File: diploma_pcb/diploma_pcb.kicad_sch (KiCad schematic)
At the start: 22 parts, among them Q1 2SC3356, Q3 2SC3356

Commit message: changes to ard, file button reader
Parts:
- Q1, Q3: footprint 2SC3356:SOT-23_MINIMOLD_REN -> 2SC3356:SOT-23_MINIMOLD_REN-M
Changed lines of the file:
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@@
 		)
 		(instances
-			(project ""
+			(project "diploma_pcb"
 				(path "/8eade999-89f4-4618-aeea-e9238b0bd165"
 					(reference "LED1")
@@
 			)
 		)
-		(property "Footprint" "2SC3356:SOT-23_MINIMOLD_REN"
+		(property "Footprint" "2SC3356:SOT-23_MINIMOLD_REN-M"
 			(at 48.895 62.865 0)
 			(effects
@@
 			)
 		)
-		(property "Footprint" "2SC3356:SOT-23_MINIMOLD_REN"
+		(property "Footprint" "2SC3356:SOT-23_MINIMOLD_REN-M"
 			(at 48.895 62.865 0)
 			(effects

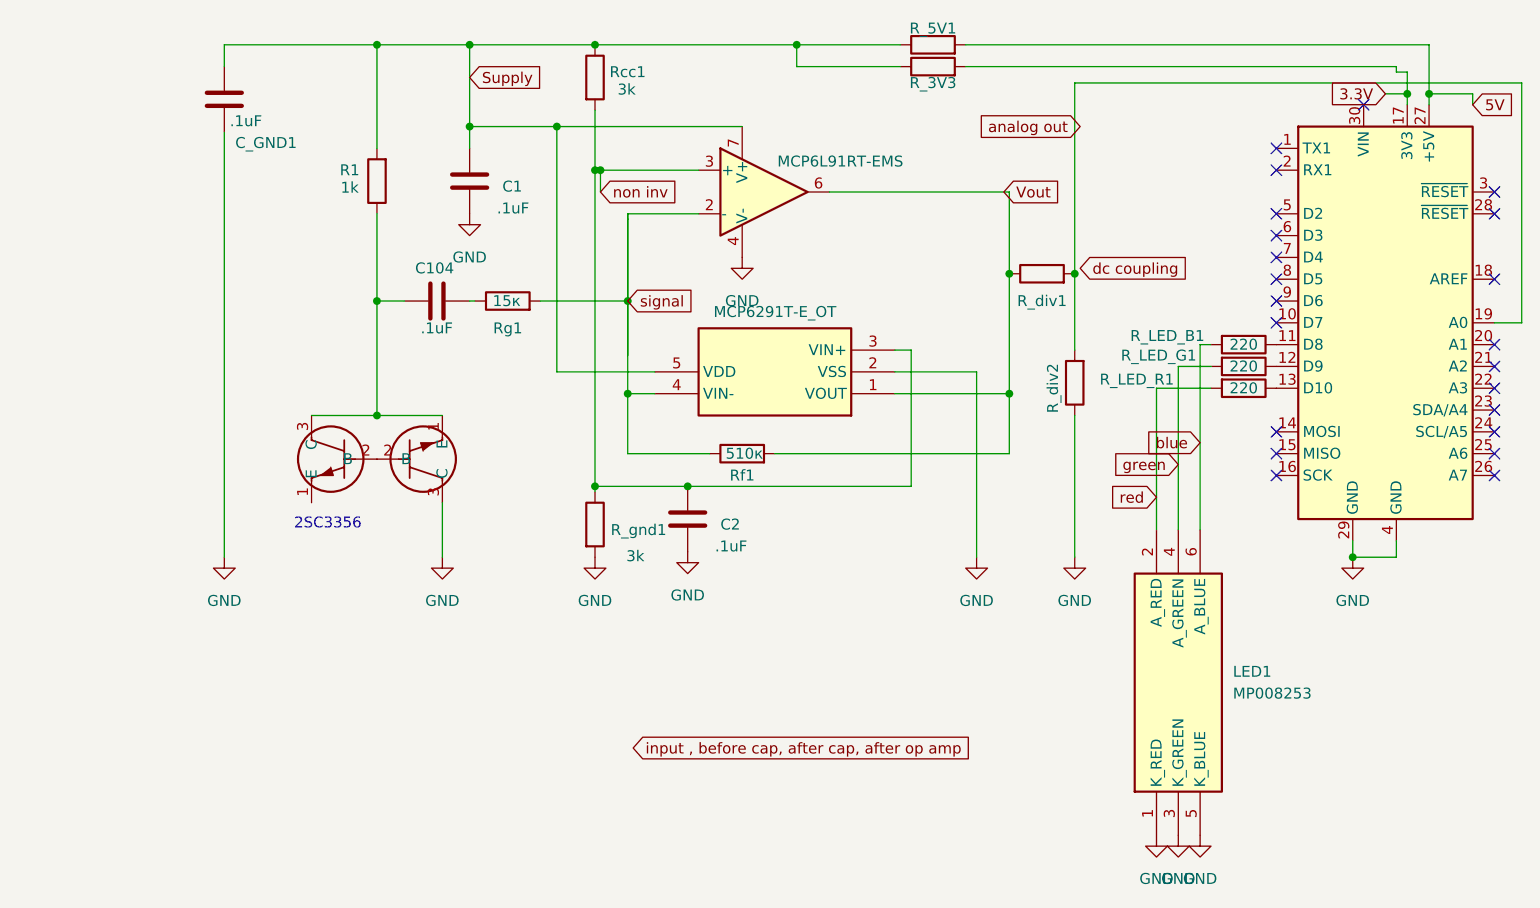
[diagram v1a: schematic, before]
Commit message: mods on PCB, Matplot, ?ard?
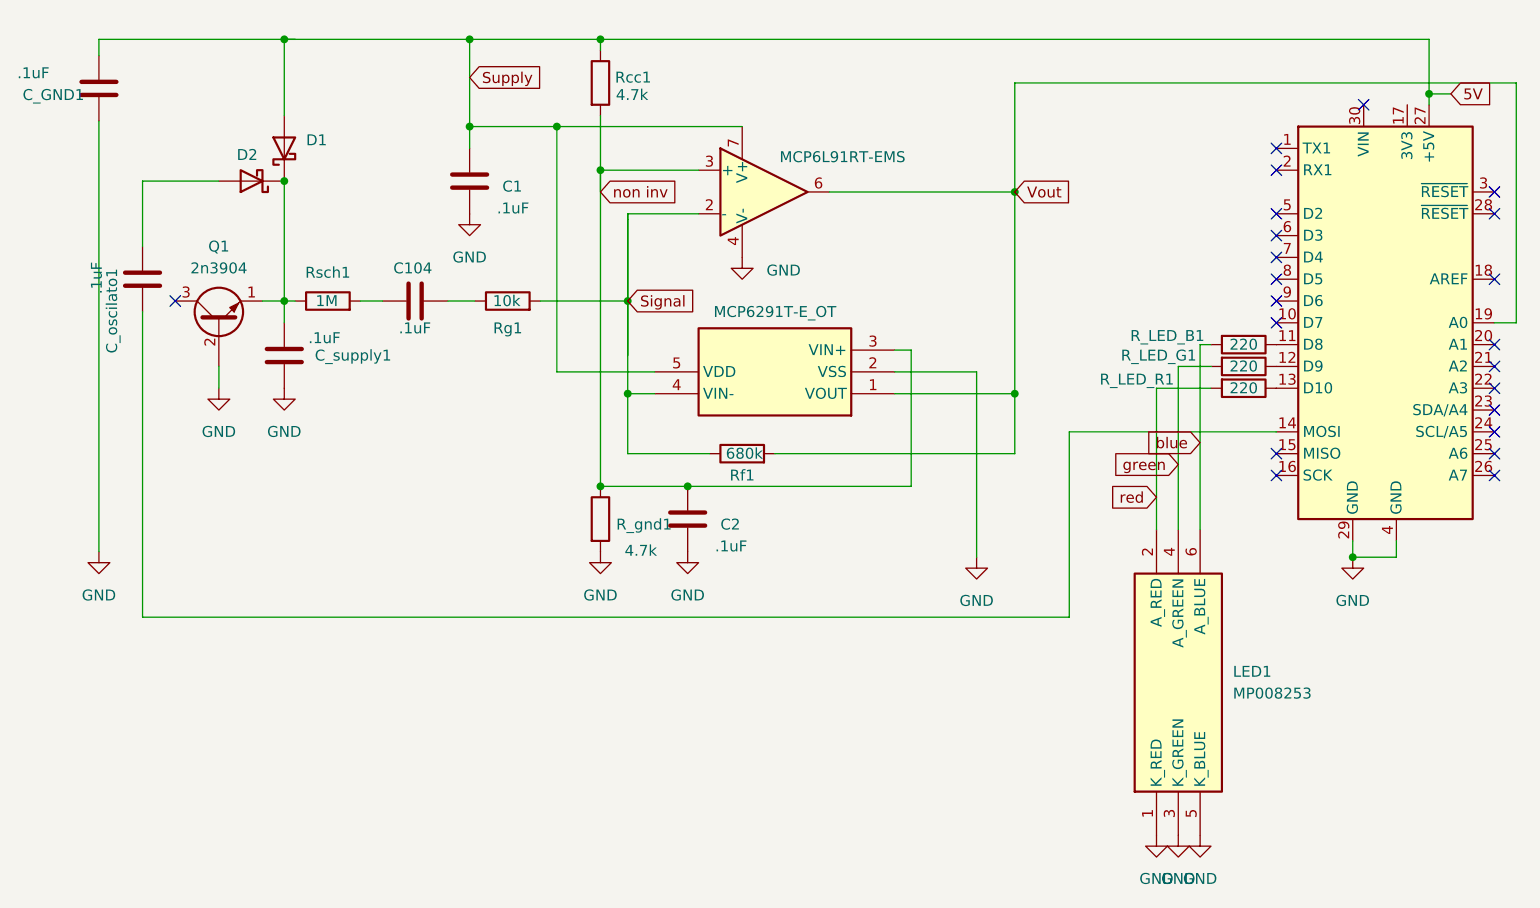
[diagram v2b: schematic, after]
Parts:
- removed Q1, Q3: 2SC3356, 2SC3356:SOT-23_MINIMOLD_REN-M, symbol 2024-08-01_13-32-15:2SC3356
- removed R1: 1k, Resistor_SMD:R_1206_3216Metric, symbol Device:R
- removed R_3V3, R_5V1, R_div1, R_div2: R, Resistor_SMD:R_1206_3216Metric, symbol Device:R
- added C_oscilato1, C_supply1: .1uF, Capacitor_SMD:C_1206_3216Metric_Pad1.33x1.80mm_HandSolder, symbol Device:C
- added D1, D2: D_Schottky, symbol Device:D_Schottky
- added Q1: 2n3904, symbol Transistor_BJT:BC107
- added Rsch1: 1M, Resistor_SMD:R_1206_3216Metric, symbol Device:R
- R_gnd1, Rcc1: value 3k -> 4.7k
- Rf1: value 510к -> 680k
- Rg1: value 15к -> 10k
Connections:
- net Supply is gone; now on net 5V: 5_pins_op_amp1.5 (VDD), 8_pin_op_amp1.7 (V+), C1.1, C_GND1.2, Rcc1.1
- net 5V: now also D1.2 (A)
- net GND: now also C_supply1.1, Q1.2 (B)
- net Vout: now also A1.19 (A0)
- net at C104.1: now also Rsch1.2
- net at A1.14 (MOSI): now also C_oscilato1.2
- net 3.3V: no longer names the net of A1.17 (3V3)
- net signal renamed Signal
- new net: C_supply1.2, D1.1 (K), D2.1 (K), Q1.1 (E), Rsch1.1
- new net: C_oscilato1.1, D2.2 (A)
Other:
- note removed: "2SC3356"
- moved on the sheet: C104, C_GND1, R_gnd1, Rcc1
